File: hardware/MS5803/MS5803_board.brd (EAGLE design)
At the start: 16 x 17 mm, 4 parts, among them U1 EM406FLAT

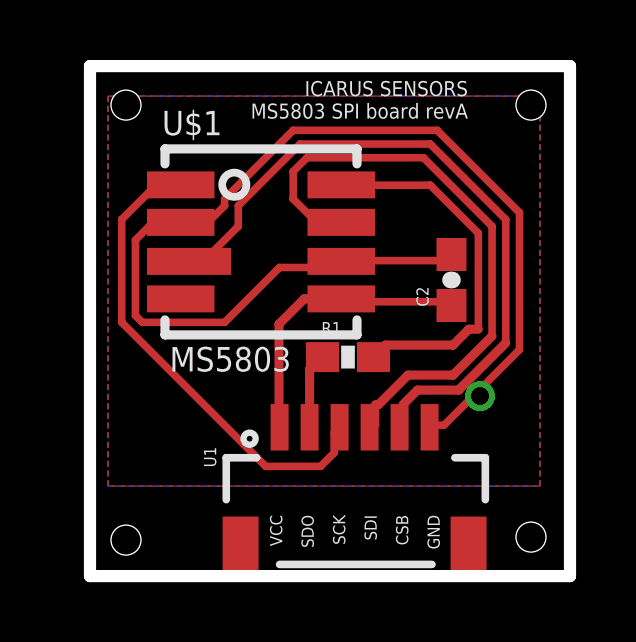
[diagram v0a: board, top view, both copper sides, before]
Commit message: MS5803
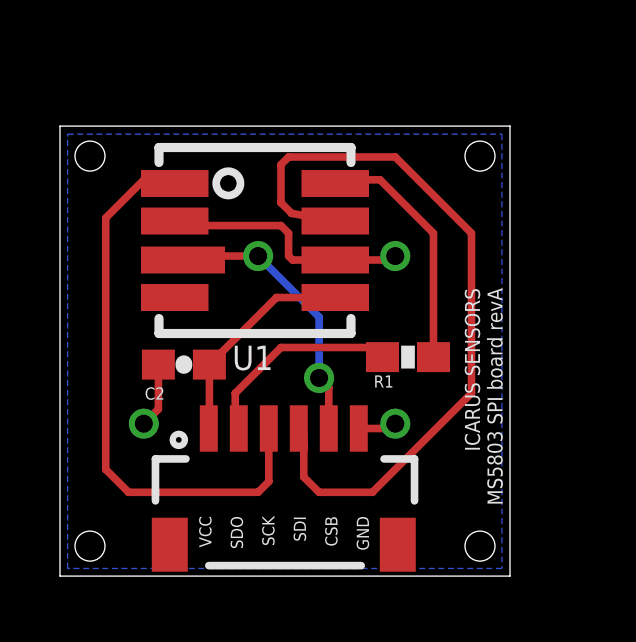
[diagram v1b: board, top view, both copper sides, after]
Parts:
- removed U$1: MS5803, icarus_sensors:MS5803
- added U2: EM406FLAT, icarus_sensors:EM406-FLAT
- C2: value 100nF -> 0.1uF
- U1: value EM406FLAT -> MS5803; device icarus_sensors:EM406-FLAT -> icarus_sensors:MS5803
- moved U1 9.74 mm to (6.50, 11.2)
- moved C2 9.36 mm to (4.13, 7.05), turned to 180 degrees
- moved R1 2.00 mm to (11.6, 7.30)
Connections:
- removed net N$1: U$1.3-CSB, U1.5
- removed net N$2: U$1.7-SDI, U1.4
- removed net N$3: U$1.1-SCLK, U1.3
- removed net N$5: R1.1, U1.2
- new net CSB: U1.3-CSB, U2.5
- new net SCK: U1.1-SCLK, U2.3
- new net SDI: U1.7-SDI, U2.4
- new net SDO: R1.1, U2.2
- net GND: now also U1.2-GND, U1.6-PS, U2.6; no longer U$1.2-GND, U$1.6-PS, U1.6
- net N$4: now also U1.8-SDO; no longer U$1.8-SDO
- net VCC: now also U1.5-VDD, U2.1; no longer U$1.5-VDD, U1.1
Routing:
- net GND: track 38.5 -> 11.9 mm, vias 1 -> 3
- net SDI: track 0.00 -> 25.4 mm
- net N$1: track 22.8 -> 0.00 mm
- net N$2: track 20.0 -> 0.00 mm
- net SCK: track 0.00 -> 18.9 mm
- net N$3: track 16.1 -> 0.00 mm
- net CSB: track 0.00 -> 9.29 mm, vias 0 -> 2
- net SDO: track 0.00 -> 6.90 mm
- net N$4: track 12.3 -> 8.19 mm
- net N$5: track 2.53 -> 0.00 mm
- net VCC: track 9.67 -> 7.27 mm
- removed copper zone on layer 1, net GND
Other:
- board size 16 x 17 mm -> 15 x 15 mm
